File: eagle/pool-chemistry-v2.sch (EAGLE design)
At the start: 17 parts, among them P10 10k, P15 15k

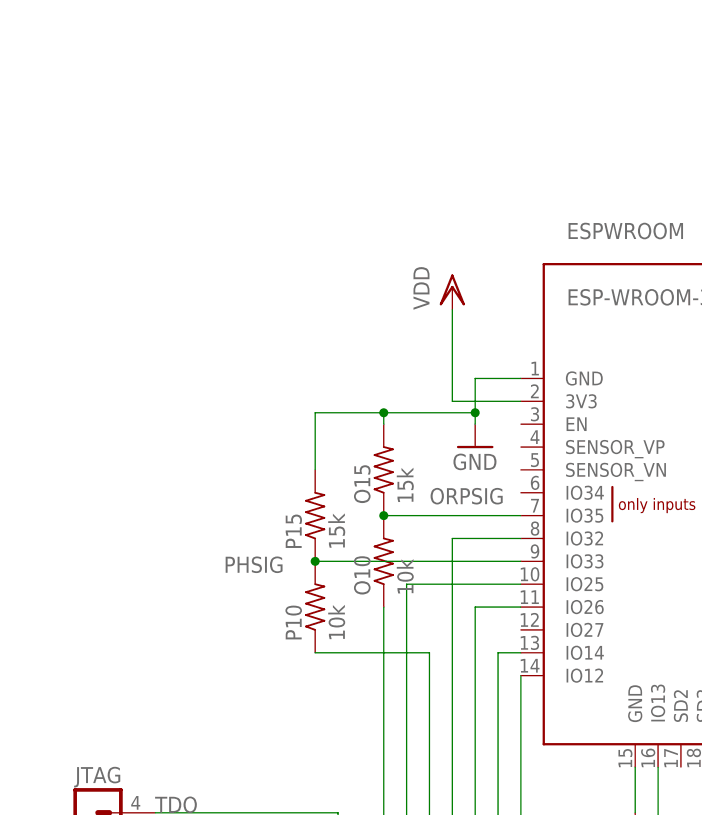
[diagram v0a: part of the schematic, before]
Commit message: added ph, orp and esp ground caps
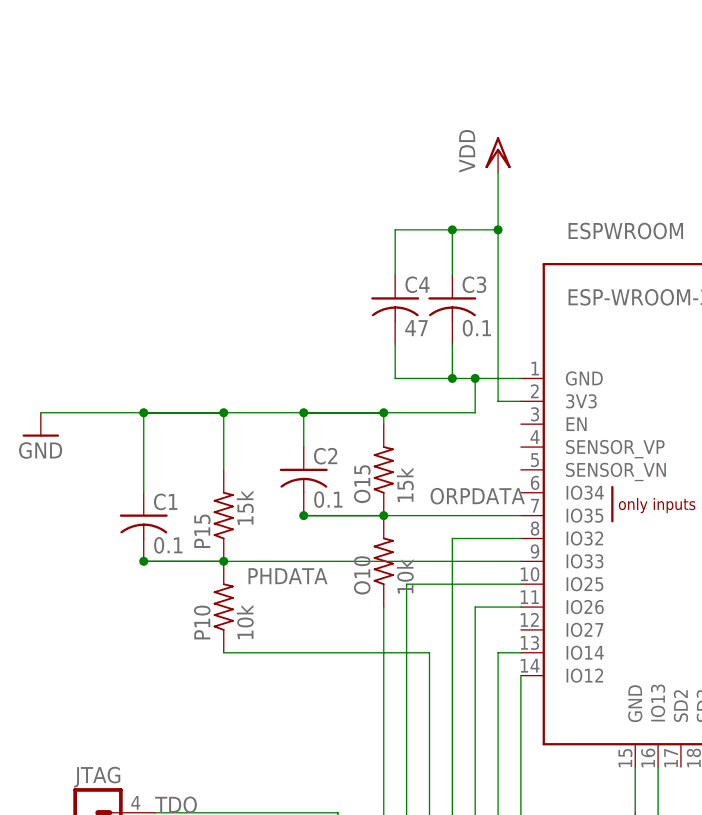
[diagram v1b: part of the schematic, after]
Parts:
- added C1, C2, C3: 0.1, rcl:C-USC1206
- added C4: 47, rcl:C-USC1206
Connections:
- new net ORPDATA: C2.2, ESPWROOM.IO35, O10.2, O15.1
- new net PHDATA: C1.2, ESPWROOM.IO33, P10.2, P15.1
- net GND: now also C1.1, C2.1, C3.2, C4.2
- net ORPSIG: no longer ESPWROOM.IO35, O10.2, O15.1
- net PHSIG: no longer ESPWROOM.IO33, P10.2, P15.1
- net VDD: now also C3.1, C4.1
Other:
- moved on the sheet: P10, P15
